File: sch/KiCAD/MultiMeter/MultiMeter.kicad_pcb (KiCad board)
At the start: 2 copper layers, 31.1 x 40.6 mm, 17 parts

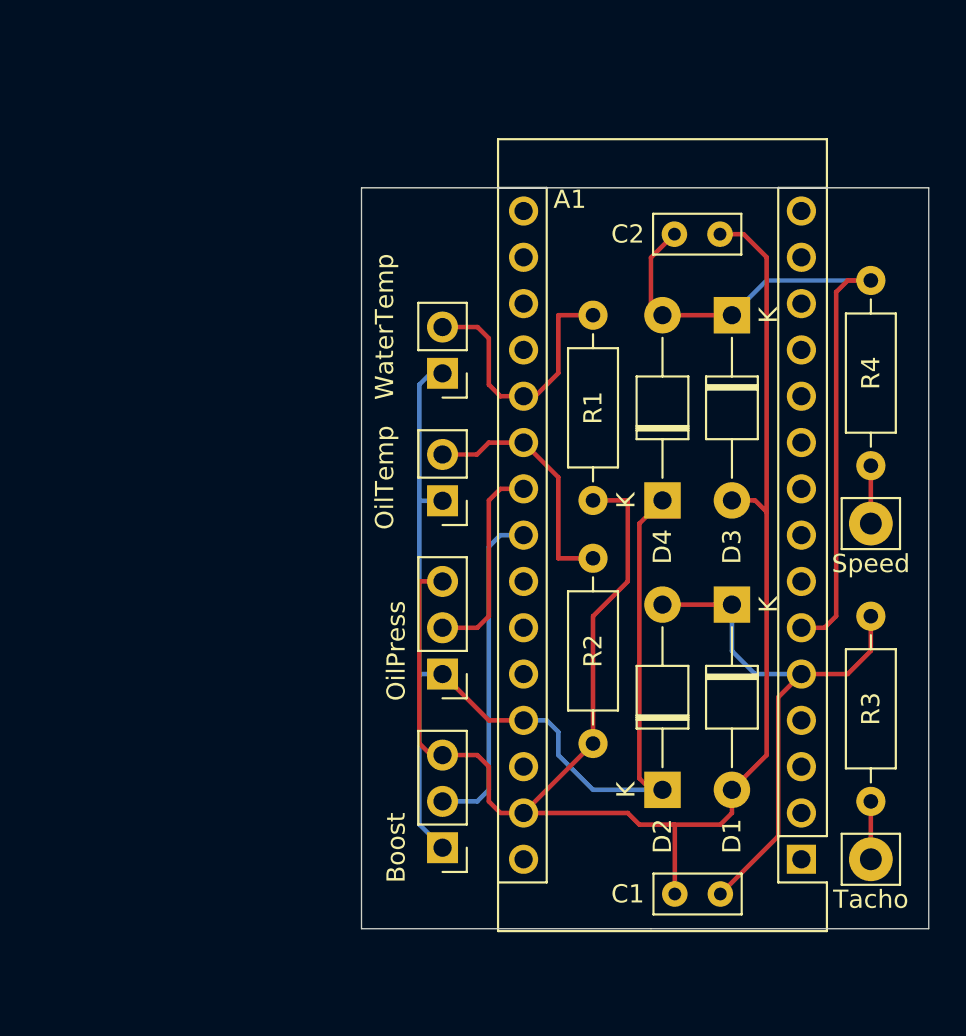
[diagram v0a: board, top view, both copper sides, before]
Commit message: 回路図データ修正
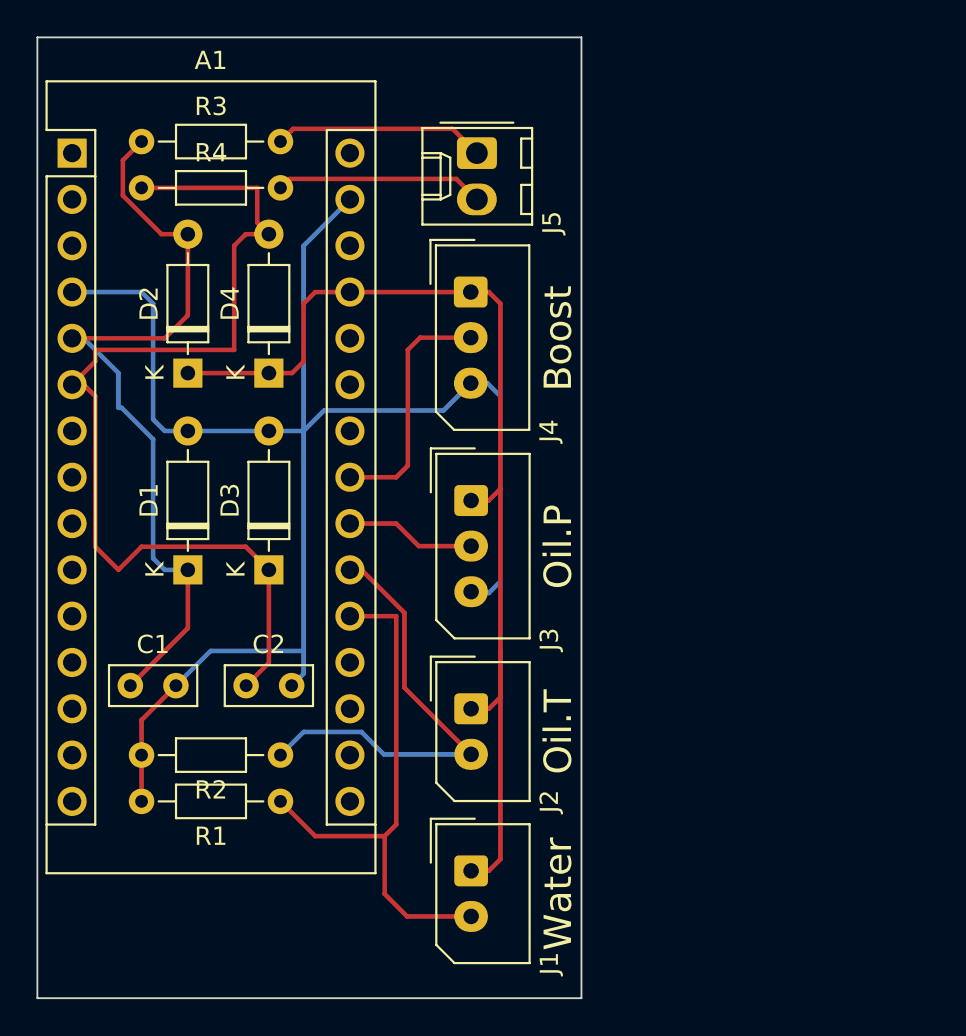
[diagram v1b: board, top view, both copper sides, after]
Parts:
- removed Boost, OilPress: PinHeader_1x03_P2.54mm_Vertical, Connector_PinHeader_2.54mm:PinHeader_1x03_P2.54mm_Vertical
- removed OilTemp, WaterTemp: PinHeader_1x02_P2.54mm_Vertical, Connector_PinHeader_2.54mm:PinHeader_1x02_P2.54mm_Vertical
- removed Speed, Tacho: Pin_D1.2mm_L11.3mm_W3.0mm_Flat, Connector_Pin:Pin_D1.2mm_L11.3mm_W3.0mm_Flat
- added J1: Conn_01x02_Male, Connector_Molex:Molex_SPOX_5267-02A_1x02_P2.50mm_Vertical, F.Cu at (64.4, 65.4)
- added J2: Conn_01x02_Male, Connector_Molex:Molex_SPOX_5267-02A_1x02_P2.50mm_Vertical, F.Cu at (64.4, 56.5)
- added J3: Conn_01x03_Male, Connector_Molex:Molex_SPOX_5267-03A_1x03_P2.50mm_Vertical, F.Cu at (64.4, 45.1)
- added J4: Conn_01x03_Male, Connector_Molex:Molex_SPOX_5267-03A_1x03_P2.50mm_Vertical, F.Cu at (64.4, 33.7)
- added J5: Conn_01x02_Female, Connector_Molex:Molex_KK-254_AE-6410-02A_1x02_P2.54mm_Vertical, F.Cu at (64.8, 26.0)
- A1: value Arduino_Nano -> Arduino_Nano_v3.x
- C1, C2: value C_Rect_L4.6mm_W2.0mm_P2.50mm_MKS02_FKP02 -> C
- D1, D2, D3, D4: value D_T-1_P10.16mm_Horizontal -> 1N4148; footprint Diode_THT:D_T-1_P10.16mm_Horizontal -> Diode_THT:D_DO-35_SOD27_P7.62mm_Horizontal
- R1, R2, R3, R4: value R_Axial_DIN0207_L6.3mm_D2.5mm_P10.16mm_Horizontal -> R; footprint Resistor_THT:R_Axial_DIN0207_L6.3mm_D2.5mm_P10.16mm_Horizontal -> Resistor_THT:R_Axial_DIN0204_L3.6mm_D1.6mm_P7.62mm_Horizontal
- moved A1 55.7 mm to (42.5, 26.0), turned to 0 degrees
- moved R3 47.7 mm to (46.4, 25.4), turned to 0 degrees
- moved R4 40.3 mm to (46.4, 27.9), turned to 0 degrees
- moved D2 34.6 mm to (48.9, 38.1)
- moved C1 34.3 mm to (45.7, 55.2), turned to 0 degrees
- moved C2 34.1 mm to (52.1, 55.2)
- moved D1 29.9 mm to (48.9, 48.9), turned to 90 degrees
- moved D3 29.0 mm to (53.3, 48.9), turned to 90 degrees
- moved R1 23.8 mm to (54.0, 61.6), turned to 180 degrees
- moved D4 22.7 mm to (53.3, 38.1)
- moved R2 17.2 mm to (54.0, 59.1), turned to 180 degrees
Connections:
- A1 pad 1: (no net) -> unconnected-(A1-Pad1)
- A1 pad 10: (no net) -> unconnected-(A1-Pad10)
- A1 pad 11: (no net) -> unconnected-(A1-Pad11)
- A1 pad 12: (no net) -> unconnected-(A1-Pad12)
- A1 pad 13: (no net) -> unconnected-(A1-Pad13)
- A1 pad 14: (no net) -> unconnected-(A1-Pad14)
- A1 pad 15: (no net) -> unconnected-(A1-Pad15)
- A1 pad 16: (no net) -> unconnected-(A1-Pad16)
- A1 pad 17: (no net) -> unconnected-(A1-Pad17)
- A1 pad 18: (no net) -> unconnected-(A1-Pad18)
- A1 pad 19: (no net) -> unconnected-(A1-Pad19)
- A1 pad 2: (no net) -> unconnected-(A1-Pad2)
- A1 pad 20: (no net) -> Net-(A1-Pad20)
- A1 pad 21: (no net) -> Net-(A1-Pad21)
- A1 pad 22: (no net) -> Net-(A1-Pad22)
- A1 pad 23: (no net) -> Net-(A1-Pad23)
- A1 pad 24: (no net) -> unconnected-(A1-Pad24)
- A1 pad 25: (no net) -> unconnected-(A1-Pad25)
- A1 pad 26: (no net) -> unconnected-(A1-Pad26)
- A1 pad 27: (no net) -> Net-(A1-Pad27)
- A1 pad 28: (no net) -> unconnected-(A1-Pad28)
- A1 pad 29: (no net) -> Net-(A1-Pad29)
- A1 pad 3: (no net) -> unconnected-(A1-Pad3)
- A1 pad 30: (no net) -> unconnected-(A1-Pad30)
- A1 pad 4: (no net) -> Net-(A1-Pad29)
- A1 pad 5: (no net) -> Net-(A1-Pad5)
- A1 pad 6: (no net) -> Net-(A1-Pad6)
- A1 pad 7: (no net) -> unconnected-(A1-Pad7)
- A1 pad 8: (no net) -> unconnected-(A1-Pad8)
- A1 pad 9: (no net) -> unconnected-(A1-Pad9)
- C1 pad 1: (no net) -> Net-(A1-Pad5)
- C1 pad 2: (no net) -> Net-(A1-Pad29)
- C2 pad 1: (no net) -> Net-(A1-Pad6)
- C2 pad 2: (no net) -> Net-(A1-Pad29)
- D1 pad 1: (no net) -> Net-(A1-Pad5)
- D1 pad 2: (no net) -> Net-(A1-Pad29)
- D2 pad 1: (no net) -> Net-(A1-Pad27)
- D2 pad 2: (no net) -> Net-(A1-Pad5)
- D3 pad 1: (no net) -> Net-(A1-Pad6)
- D3 pad 2: (no net) -> Net-(A1-Pad29)
- D4 pad 1: (no net) -> Net-(A1-Pad27)
- D4 pad 2: (no net) -> Net-(A1-Pad6)
- R1 pad 1: (no net) -> Net-(A1-Pad20)
- R1 pad 2: (no net) -> Net-(A1-Pad29)
- R2 pad 1: (no net) -> Net-(A1-Pad21)
- R2 pad 2: (no net) -> Net-(A1-Pad29)
- R3 pad 1: (no net) -> Net-(A1-Pad5)
- R3 pad 2: (no net) -> Net-(J5-Pad1)
- R4 pad 1: (no net) -> Net-(A1-Pad6)
- R4 pad 2: (no net) -> Net-(J5-Pad2)
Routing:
- net (no net): track 290.2 -> 0.00 mm
- net Net-(A1-Pad29): track 0.00 -> 86.6 mm
- net Net-(A1-Pad27): track 0.00 -> 59.7 mm
- net Net-(A1-Pad6): track 0.00 -> 54.2 mm
- net Net-(A1-Pad5): track 0.00 -> 42.7 mm
- net Net-(A1-Pad20): track 0.00 -> 29.8 mm
- net Net-(A1-Pad21): track 0.00 -> 24.1 mm
- net Net-(A1-Pad23): track 0.00 -> 13.5 mm
- net Net-(J5-Pad1): track 0.00 -> 11.6 mm
- net Net-(J5-Pad2): track 0.00 -> 11.4 mm
- net Net-(A1-Pad22): track 0.00 -> 7.16 mm
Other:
- board size 31.1 x 40.6 mm -> 29.8 x 52.7 mm
- board text added: "2022/09/13"
- board text added: "Boost"
- board text added: "Oil.P"
- board text added: "Oil.T"
- board text added: "Water"
- board text removed: "2022/08/18"
- board text removed: "USB"
